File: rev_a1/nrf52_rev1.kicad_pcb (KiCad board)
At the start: 2 copper layers, 99.1 x 48.3 mm, 28 parts, among them P1 CONN_01X18, P2 CONN_01X18, P3 USB_OTG, P4 I2C_OLED, U1 nRF52832, U2 CP2102, U3 LT1129CST-3.3, Y1 32K, Y2 32M

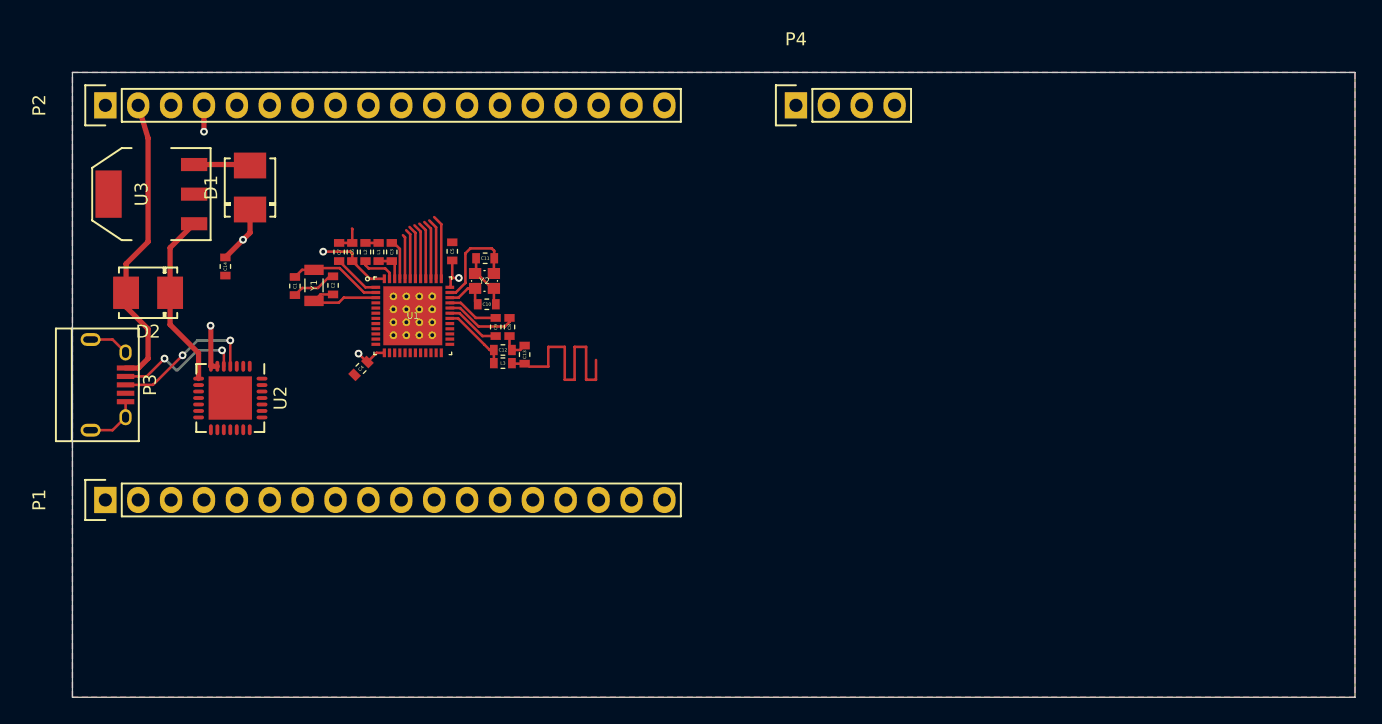
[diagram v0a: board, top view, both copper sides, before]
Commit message: Wiiip
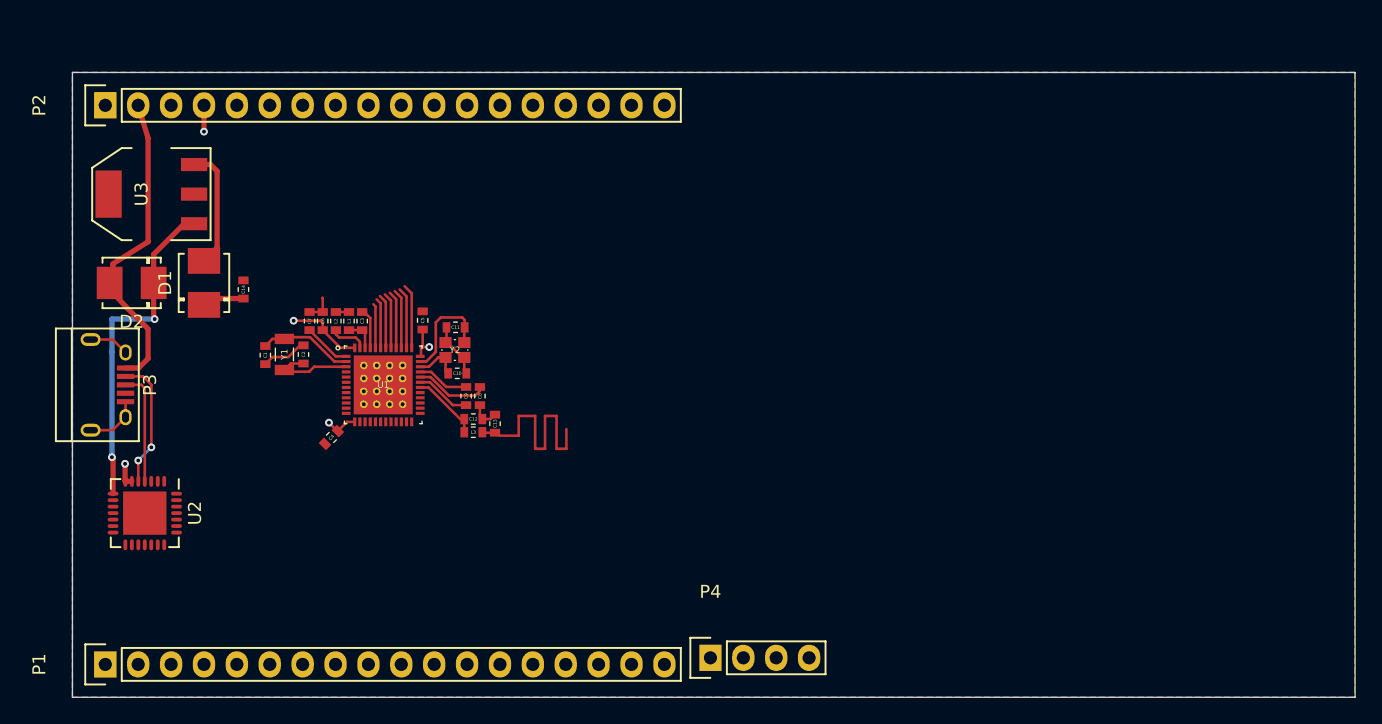
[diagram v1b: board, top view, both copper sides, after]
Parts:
- moved P4 43.2 mm to (74.7, 70.6)
- moved P1 12.7 mm to (27.9, 71.1)
- moved U2 11.1 mm to (31.0, 59.4)
- moved D1 8.18 mm to (35.6, 41.7)
- moved C11 5.80 mm to (55.0, 45.1)
- moved C13 5.80 mm to (58.0, 52.5)
- moved C2 5.80 mm to (43.2, 47.2)
- moved C3 5.80 mm to (47.8, 44.6)
- moved C5 5.80 mm to (52.5, 44.6)
- moved C6 5.80 mm to (44.7, 44.6)
- moved C7 5.80 mm to (43.7, 44.6)
- moved L1 5.80 mm to (46.8, 44.6)
- moved L2 5.80 mm to (45.7, 44.6)
- moved L3 5.80 mm to (56.4, 53.2)
- moved U1 5.80 mm to (49.4, 49.5)
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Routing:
- net +5V: track 13.6 -> 27.7 mm, vias 0 -> 2
- net Net-(D1-Pad2): track 4.57 -> 9.35 mm
- net +3V3: track 21.7 -> 18.6 mm, vias 6 -> 5
- net USB_D+: track 11.5 -> 8.79 mm, vias 2 -> 0
- net 5V_IN: track 24.7 -> 26.4 mm
